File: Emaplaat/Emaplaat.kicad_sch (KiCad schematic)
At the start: 15 parts, among them IC1 ESP32-S3-WROOM-2-N32R16V, IC13 74HC595PW-Q100,118, IC7 74HC595PW-Q100,118

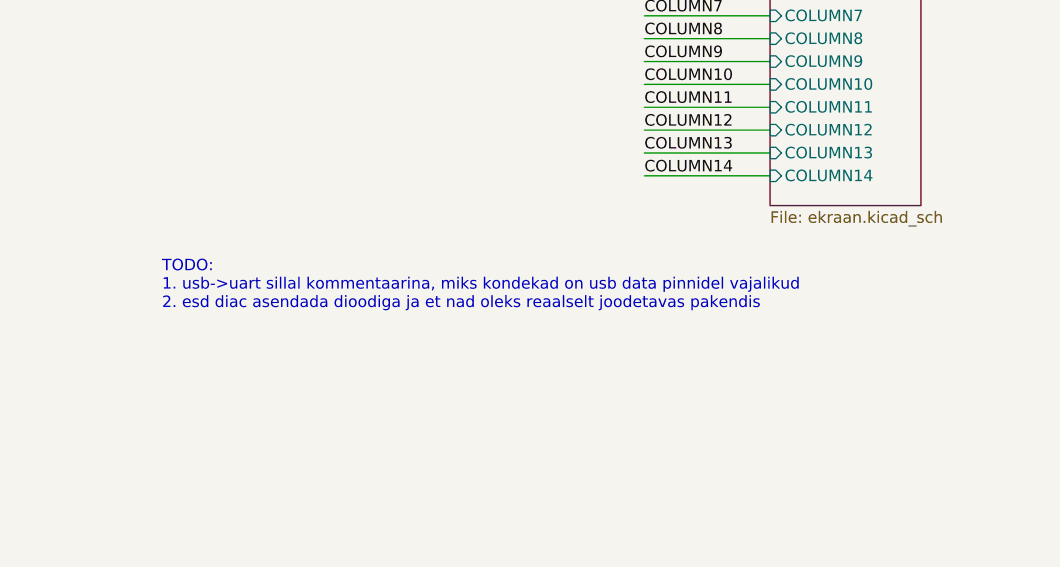
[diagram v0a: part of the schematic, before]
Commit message: Kaareli kolmas tagasiside
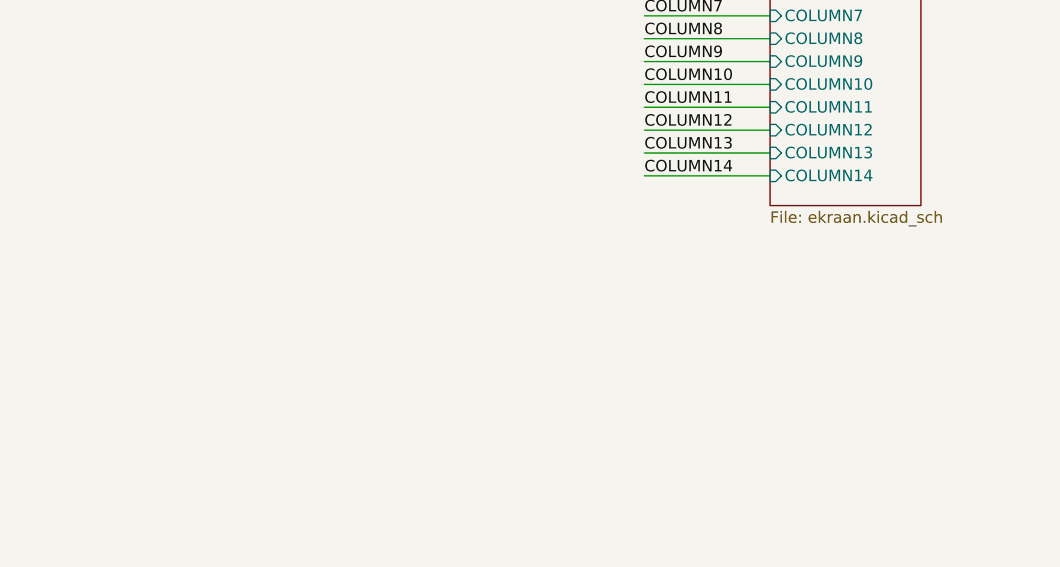
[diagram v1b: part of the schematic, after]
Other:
- note removed: "TODO: 1. usb->uart sillal kommentaarina, miks kondekad on usb data pinnidel vajalikud 2. esd diac asendada dioodiga ja et nad oleks reaalselt joodetavas pakendis"
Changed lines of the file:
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@@
-		)
-	)
-	(text "TODO:\n1. usb->uart sillal kommentaarina, miks kondekad on usb data pinnidel vajalikud\n2. esd diac asendada dioodiga ja et nad oleks reaalselt joodetavas pakendis\n"
-		(exclude_from_sim no)
-		(at 178.816 144.272 0)
-		(effects
-			(font
-				(size 1.27 1.27)
-			)
-			(justify left)
 		)
 	)
